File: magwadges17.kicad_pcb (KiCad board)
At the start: 2 copper layers, 156 x 89.8 mm, 52 parts, among them J1 PGM, J2 JACK_2P, U1 ATTINY861A-SU

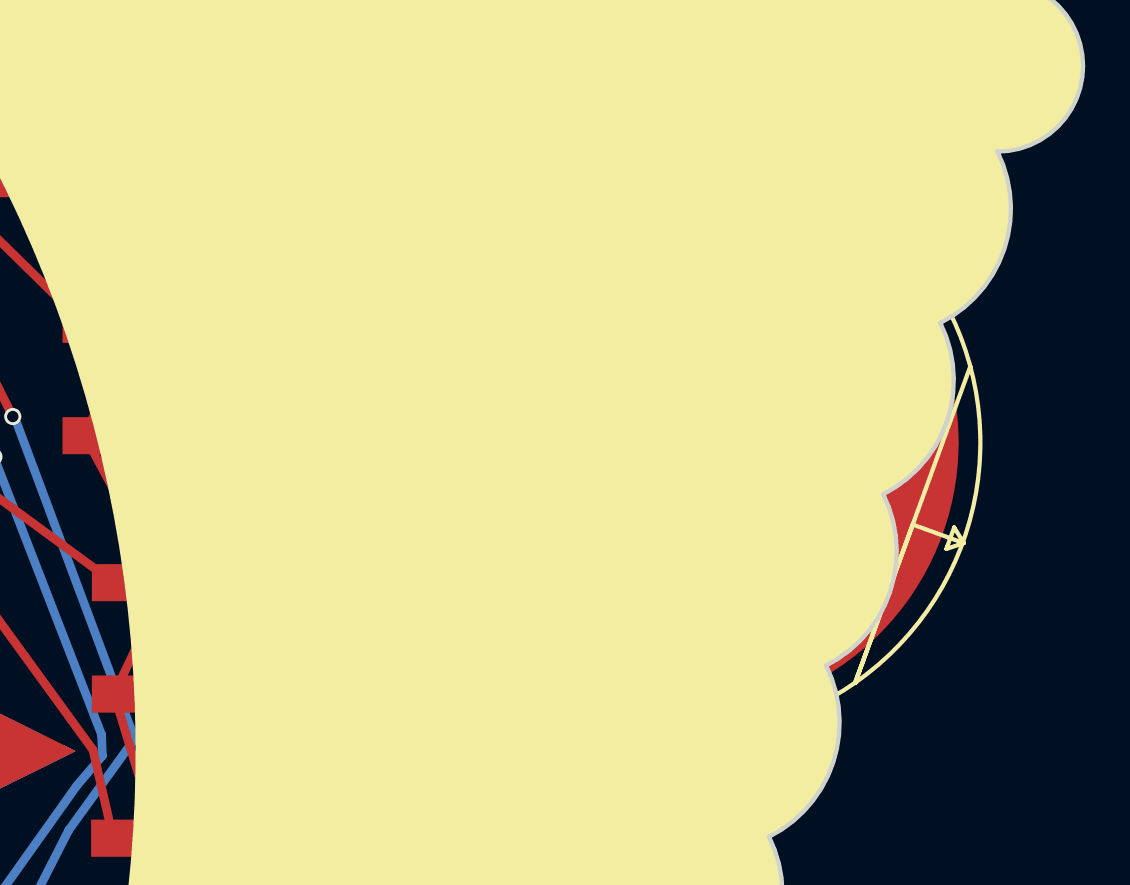
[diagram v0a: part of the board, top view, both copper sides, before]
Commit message: final plots as they were sent.
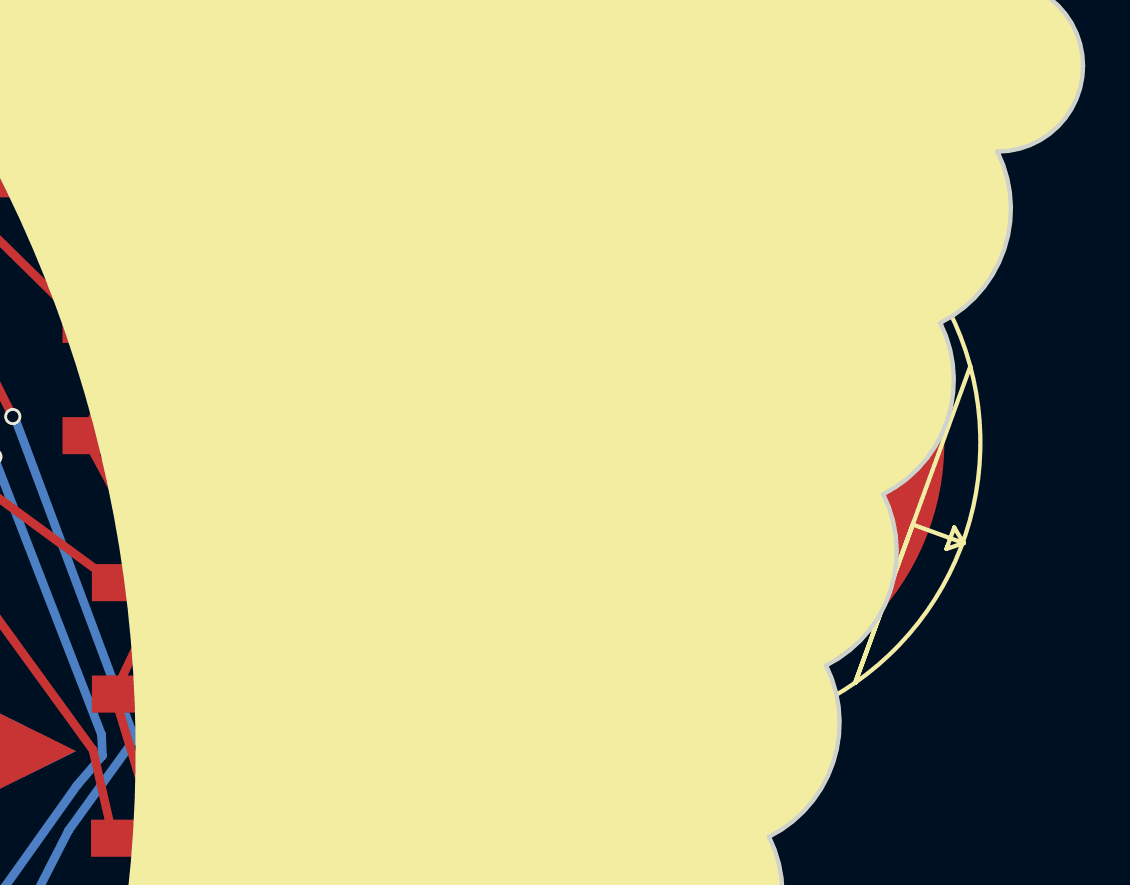
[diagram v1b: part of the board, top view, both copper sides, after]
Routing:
- net (no net): track 0.00 -> 6.50 mm
